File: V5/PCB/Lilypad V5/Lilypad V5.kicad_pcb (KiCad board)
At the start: 2 copper layers, 46.3 x 51.3 mm, 58 parts, among them J1 USB-C, J2 TRRS, SW1 BTN_RESET, SW2 BTN_USER, SW3 BTN_BOOT, U1 SRV05-4, U2 M3406, U3 BQ21040, U4 SRV05-4, U5 ESP32-C3-MINI-1-N4, U6 BMI270

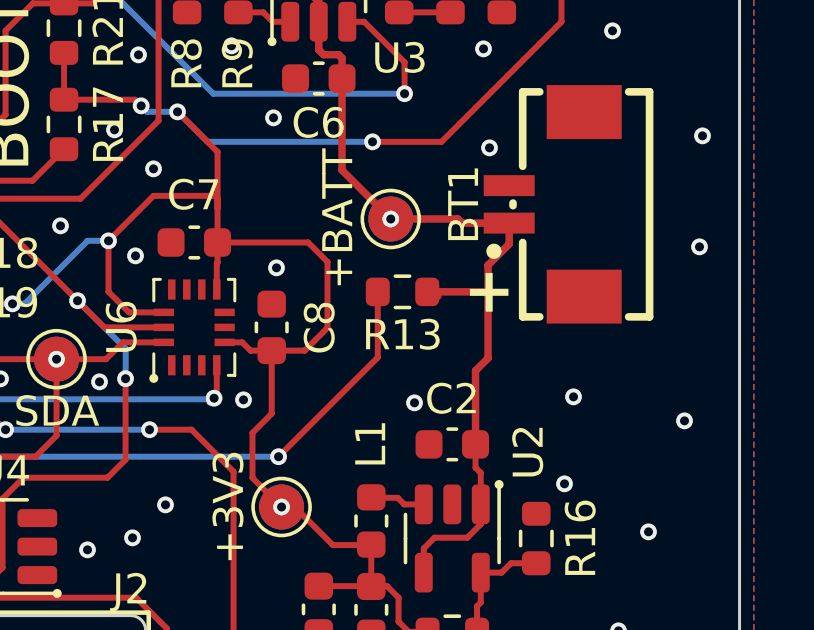
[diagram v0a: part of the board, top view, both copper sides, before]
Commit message: V5 CAD started
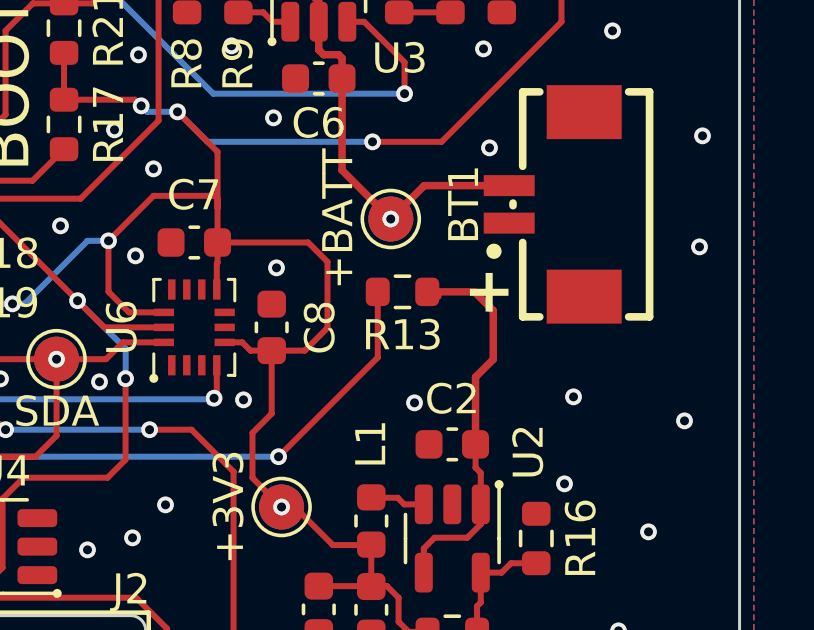
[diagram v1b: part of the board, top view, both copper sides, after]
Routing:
- net +BATT: track 47.7 -> 45.3 mm
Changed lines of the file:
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@@
 		)
 		(pad "1" smd rect
-			(at -0.624968 -1.250064 90)
+			(at 0.624968 -1.250064 90)
 			(size 0.7 1.7)
 			(layers "F.Cu" "F.Paste" "F.Mask")
@@
 		)
 		(pad "2" smd rect
-			(at 0.624968 -1.250064 90)
+			(at -0.624968 -1.250064 90)
 			(size 0.7 1.7)
 			(layers "F.Cu" "F.Paste" "F.Mask")
@@
 	)
 	(segment
-		(start 125.384459 99.546949)
-		(end 127.009458 101.17195)
+		(start 129.834459 106.440541)
+		(end 130.425 105.85)
 		(width 0.25)
 		(layer "F.Cu")
@@
 	)
 	(segment
-		(start 125.384458 96.488948)
-		(end 125.384459 95.810977)
-		(width 0.25)
-		(layer "F.Cu")
-		(net 12)
-	)
-	(segment
-		(start 130.956332 101.308703)
-		(end 130.956332 102.007137)
+		(start 125.384459 99.546949)
+		(end 127.009458 101.17195)
 		(width 0.25)
 		(layer "F.Cu")
@@
 	)
 	(segment
-		(start 130.147509 103.6)
-		(end 128.225 103.6)
+		(start 125.384458 96.488948)
+		(end 125.384459 95.810977)
 		(width 0.25)
 		(layer "F.Cu")
@@
 	)
 	(segment
-		(start 130.956332 102.007137)
-		(end 130.25146 102.712008)
+		(start 130.425 104.225)
+		(end 129.8 103.6)
 		(width 0.25)
 		(layer "F.Cu")
@@
 	)
 	(segment
-		(start 130.251459 103.70395)
-		(end 130.147509 103.6)
-		(width 0.25)
-		(layer "F.Cu")
-		(net 12)
-	)
-	(segment
 		(start 130.009459 110.684448)
 		(end 130.009458 109.635979)
@@
 	)
 	(segment
-		(start 130.251459 103.70395)
-		(end 130.251462 105.812008)
-		(width 0.25)
-		(layer "F.Cu")
-		(net 12)
-	)
-	(segment
-		(start 130.251462 105.812008)
-		(end 129.834459 106.229011)
-		(width 0.25)
-		(layer "F.Cu")
-		(net 12)
-	)
-	(segment
-		(start 129.834459 106.229011)
-		(end 129.834459 108.684448)
-		(width 0.25)
-		(layer "F.Cu")
-		(net 12)
-	)
-	(segment
 		(start 122.769906 93.097901)
 		(end 122.769906 91.472434)
@@
 	)
 	(segment
-		(start 129.382184 101.308702)
-		(end 130.956332 101.308703)
-		(width 0.25)
-		(layer "F.Cu")
-		(net 12)
-	)
-	(segment
 		(start 128.109459 112.15401)
 		(end 128.468475 111.794994)
@@
 	)
 	(segment
-		(start 129.245432 101.17195)
-		(end 129.382184 101.308702)
+		(start 127.009458 101.17195)
+		(end 128.122641 100.058767)
 		(width 0.25)
 		(layer "F.Cu")
@@
 	)
 	(segment
-		(start 130.25146 102.712008)
-		(end 130.251459 103.70395)
+		(start 130.425 105.85)
+		(end 130.425 104.225)
 		(width 0.25)
 		(layer "F.Cu")
@@
 	)
 	(segment
-		(start 127.009458 101.17195)
-		(end 129.245432 101.17195)
+		(start 129.8 103.6)
+		(end 128.225 103.6)
 		(width 0.25)
 		(layer "F.Cu")
@@
 	)
 	(segment
+		(start 128.122641 100.058767)
+		(end 130.956332 100.058767)
+		(width 0.25)
+		(layer "F.Cu")
+		(net 12)
+	)
+	(segment
 		(start 125.384458 96.488948)
 		(end 125.384459 99.546949)
 		(width 0.25)
 		(layer "F.Cu")
+		(net 12)
+	)
+	(segment
+		(start 129.834459 108.684448)
+		(end 129.834459 106.440541)
+		(width 0.25)
+		(layer "F.Cu")
